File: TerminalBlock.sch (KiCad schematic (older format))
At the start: 2 parts, among them P4 12 Pin Terminal Block, P5 3 Pin TB

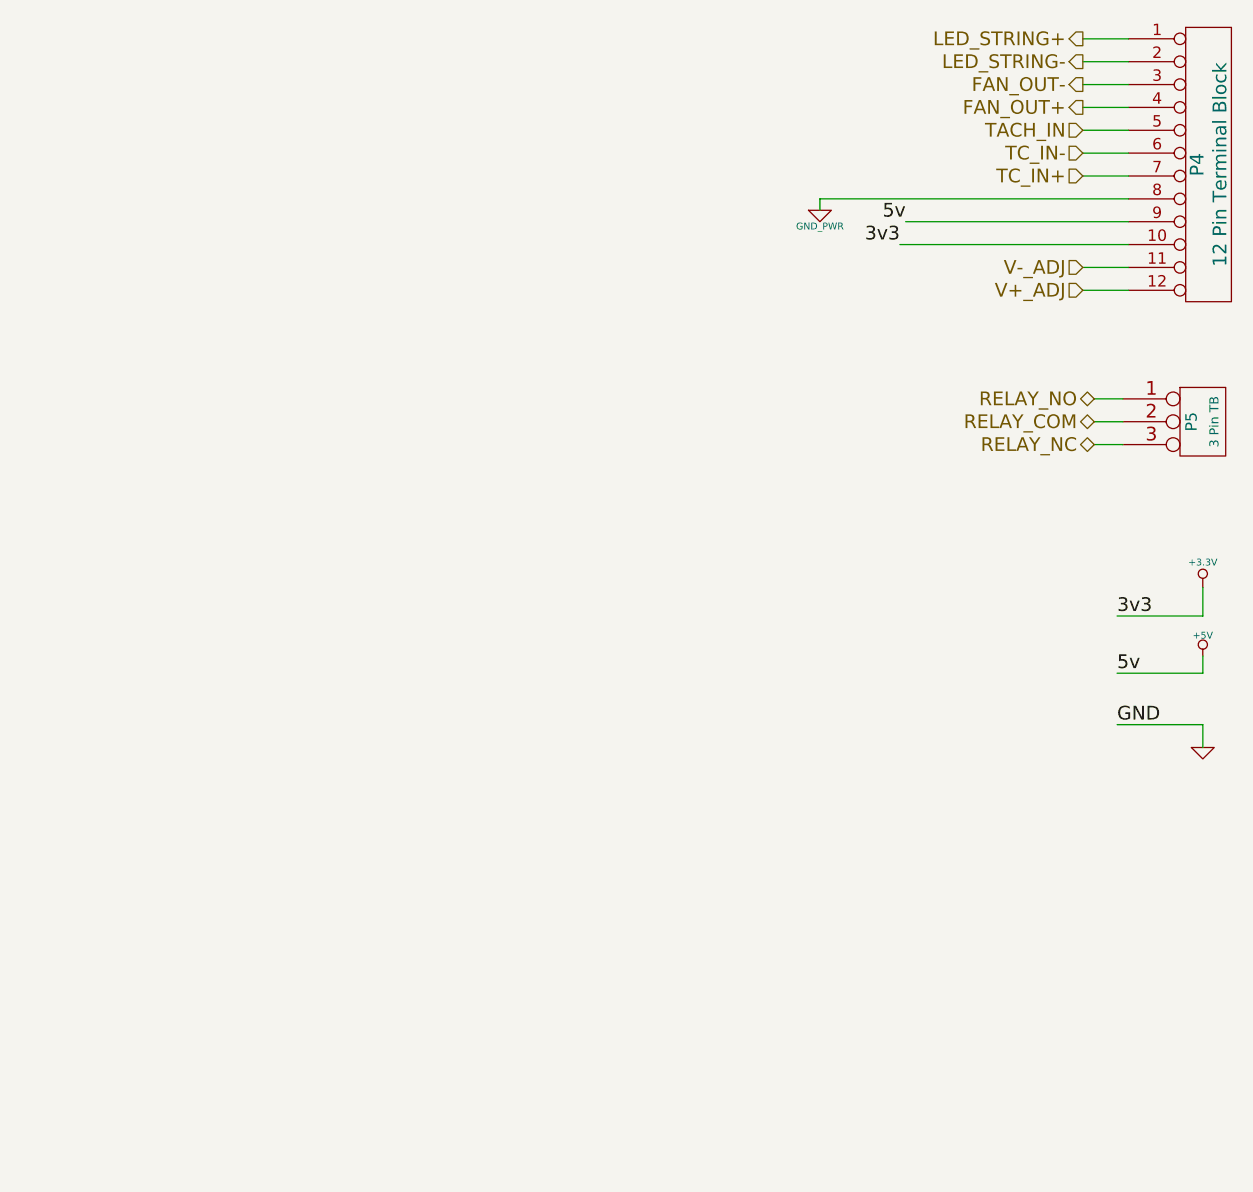
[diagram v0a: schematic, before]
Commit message: Layout Work Session 6
Pulled from CE
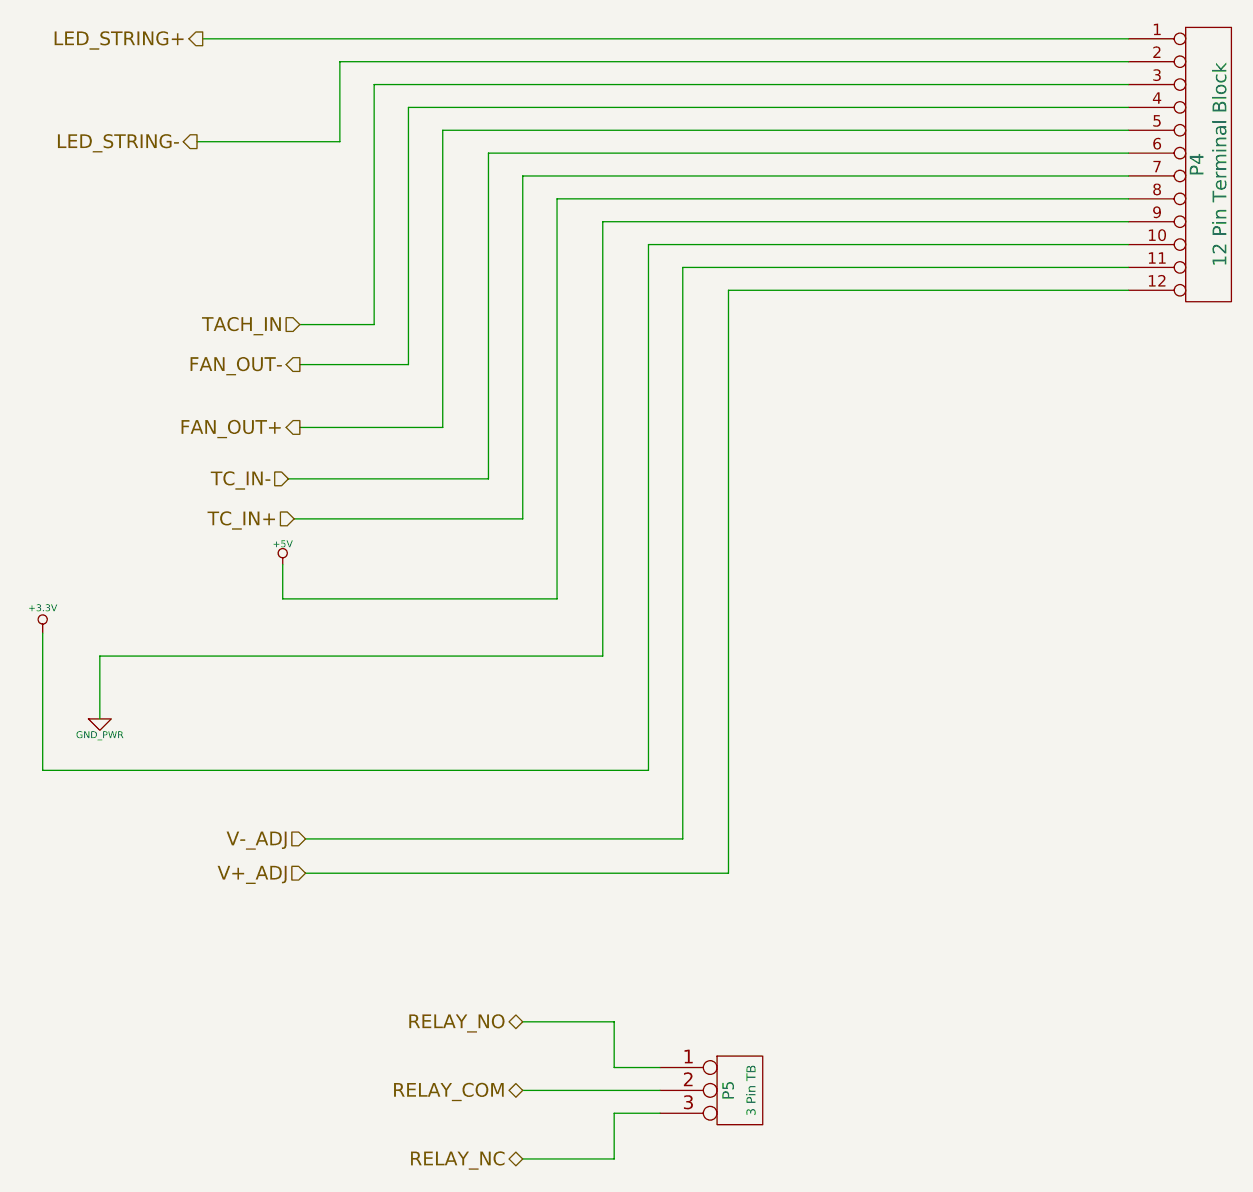
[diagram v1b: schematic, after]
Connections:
- net +5V: now also P4.8 (P8); no longer P4.9 (P9)
- net FAN_OUT+: now also P4.5 (P5); no longer P4.4 (P4)
- net FAN_OUT-: now also P4.4 (P4); no longer P4.3 (P3)
- net GND_PWR: now also P4.9 (P9); no longer P4.8 (P8)
- net TACH_IN: now also P4.3 (P3); no longer P4.5 (P5)
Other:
- moved on the sheet: P5
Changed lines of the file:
@@
-EESchema Schematic File Version 2
+EESchema Schematic File Version 2  date 11/10/2013 9:27:17 PM
 LIBS:power
 LIBS:device
@@
 LIBS:valves
 LIBS:BenchBuddy
-LIBS:arduino_shieldsNCL
 LIBS:BenchBuddy-cache
-EELAYER 24 0
+EELAYER 27 0
 EELAYER END
 $Descr A4 11693 8268
@@
 Sheet 7 9
 Title ""
-Date "2 nov 2013"
+Date "11 nov 2013"
 Rev ""
 Comp ""
@@
 Comment4 ""
 $EndDescr
-Text HLabel 5300 2000 0    60   Input ~ 0
+Text HLabel 1900 4550 0    60   Input ~ 0
 V+_ADJ
-Text HLabel 5300 1900 0    60   Input ~ 0
+Text HLabel 1900 4400 0    60   Input ~ 0
 V-_ADJ
-Text HLabel 5300 1200 0    60   Output ~ 0
+Text HLabel 1875 2600 0    60   Output ~ 0
 FAN_OUT+
-Text HLabel 5300 1100 0    60   Output ~ 0
+Text HLabel 1875 2325 0    60   Output ~ 0
 FAN_OUT-
-Text HLabel 5300 1300 0    60   Input ~ 0
+Text HLabel 1875 2150 0    60   Input ~ 0
 TACH_IN
-Text HLabel 5300 900  0    60   Output ~ 0
+Text HLabel 1450 900  0    60   Output ~ 0
 LED_STRING+
-Text HLabel 5300 1000 0    60   Output ~ 0
+Text HLabel 1425 1350 0    60   Output ~ 0
 LED_STRING-
-Text HLabel 5300 1500 0    60   Input ~ 0
+Text HLabel 1850 3000 0    60   Input ~ 0
 TC_IN+
-Text HLabel 5300 1400 0    60   Input ~ 0
+Text HLabel 1825 2825 0    60   Input ~ 0
 TC_IN-
-Text HLabel 5350 2575 0    60   BiDi ~ 0
+Text HLabel 2850 5500 0    60   BiDi ~ 0
 RELAY_COM
-Text HLabel 5350 2475 0    60   BiDi ~ 0
+Text HLabel 2850 5200 0    60   BiDi ~ 0
 RELAY_NO
-Text HLabel 5350 2675 0    60   BiDi ~ 0
+Text HLabel 2850 5800 0    60   BiDi ~ 0
 RELAY_NC
 $Comp
-L +3.3V #PWR038
+L +3.3V #PWR44
 U 1 1 523FFDA7
-P 5825 3300
-F 0 "#PWR038" H 5825 3260 30  0001 C CNN
-F 1 "+3.3V" H 5825 3410 30  0000 C CNN
-F 2 "~" H 5825 3300 60  0000 C CNN
-F 3 "~" H 5825 3300 60  0000 C CNN
-	1    5825 3300
-	1    0    0    -1
-$EndComp
-$Comp
-L +5V #PWR039
+P 750 3500
+F 0 "#PWR44" H 750 3460 30  0001 C CNN
+F 1 "+3.3V" H 750 3610 30  0000 C CNN
+F 2 "~" H 750 3500 60  0000 C CNN
+F 3 "~" H 750 3500 60  0000 C CNN
+	1    750  3500
+	1    0    0    -1
+$EndComp
+$Comp
+L +5V #PWR45
 U 1 1 523FFDB6
-P 5825 3600
-F 0 "#PWR039" H 5825 3690 20  0001 C CNN
-F 1 "+5V" H 5825 3690 30  0000 C CNN
-F 2 "~" H 5825 3600 60  0000 C CNN
-F 3 "~" H 5825 3600 60  0000 C CNN
-	1    5825 3600
+P 1800 3200
+F 0 "#PWR45" H 1800 3290 20  0001 C CNN
+F 1 "+5V" H 1800 3290 30  0000 C CNN
+F 2 "~" H 1800 3200 60  0000 C CNN
+F 3 "~" H 1800 3200 60  0000 C CNN
+	1    1800 3200
 	1    0    0    -1
 $EndComp
@@
 	1    0    0    -1
 $EndComp
+Wire Wire Line
+	1425 1350 2050 1350
+Wire Wire Line
+	2050 1350 2050 1000
+Wire Wire Line
+	2050 1000 5500 1000
+Wire Wire Line
+	2200 1100 5500 1100
+Wire Wire Line
+	2200 1100 2200 2150
+Wire Wire Line
+	2350 1200 2350 2325
+Wire Wire Line
+	2350 1200 5500 1200
+Wire Wire Line
+	5500 1300 2500 1300
+Wire Wire Line
+	2500 1300 2500 2600
+Wire Wire Line
+	2700 2825 2700 1400
+Wire Wire Line
+	2700 1400 5500 1400
+Wire Wire Line
+	1800 3350 3000 3350
+Wire Wire Line
+	1000 3600 3200 3600
+Wire Wire Line
+	750  4100 3400 4100
+Wire Wire Line
+	2850 1500 2850 3000
+Wire Wire Line
+	2850 1500 5500 1500
+Wire Wire Line
+	5500 1600 3000 1600
+Wire Wire Line
+	3000 1600 3000 3350
+Wire Wire Line
+	3200 3600 3200 1700
+Wire Wire Line
+	3200 1700 5500 1700
+Wire Wire Line
+	5500 1800 3400 1800
+Wire Wire Line
+	3400 1800 3400 4100
+Wire Wire Line
+	1900 4400 3550 4400
+Wire Wire Line
+	3550 4400 3550 1900
+Wire Wire Line
+	3550 1900 5500 1900
+Wire Wire Line
+	5500 2000 3750 2000
+Wire Wire Line
+	3750 2000 3750 4550
+Wire Wire Line
+	3750 4550 1900 4550
 $Comp
 L CONN_3 P5
 U 1 1 5258AA07
-P 5825 2575
-F 0 "P5" V 5775 2575 50  0000 C CNN
-F 1 "3 Pin TB" V 5875 2575 40  0000 C CNN
-F 2 "" H 5825 2575 60  0000 C CNN
-F 3 "" H 5825 2575 60  0000 C CNN
-F 4 "Phoenix" H 5825 2575 60  0001 C CNN "MFG Name"
-F 5 "1935174" H 5825 2575 60  0001 C CNN "MFG Part Number"
-	1    5825 2575
-	1    0    0    -1
-$EndComp
-Wire Wire Line
-	5475 2575 5350 2575
-$Comp
-L GND #PWR040
-U 1 1 523FFDC5
-P 5825 4000
-F 0 "#PWR040" H 5825 4000 30  0001 C CNN
-F 1 "GND" H 5825 3930 30  0001 C CNN
-F 2 "~" H 5825 4000 60  0000 C CNN
-F 3 "~" H 5825 4000 60  0000 C CNN
-	1    5825 4000
-	1    0    0    -1
-$EndComp
-Wire Wire Line
-	5350 2475 5475 2475
-Wire Wire Line
-	5350 2675 5475 2675
-Wire Wire Line
-	5825 3300 5825 3425
-Wire Wire Line
-	5825 3425 5450 3425
-Text Label 5450 3425 0    60   ~ 0
-3v3
-Wire Wire Line
-	5825 3600 5825 3675
-Wire Wire Line
-	5825 3675 5450 3675
-Wire Wire Line
-	5825 4000 5825 3900
-Wire Wire Line
-	5825 3900 5450 3900
-Text Label 5450 3675 0    60   ~ 0
-5v
-Text Label 5450 3900 0    60   ~ 0
-GND
-Wire Wire Line
-	5300 2000 5500 2000
-Wire Wire Line
-	5500 1900 5300 1900
-Wire Wire Line
-	4500 1800 5500 1800
-Wire Wire Line
-	4525 1700 5500 1700
-Wire Wire Line
-	4150 1600 5500 1600
-Wire Wire Line
-	5500 1300 5300 1300
-Wire Wire Line
-	5500 900  5300 900
-Wire Wire Line
-	5300 1000 5500 1000
-Wire Wire Line
-	5500 1200 5300 1200
-Wire Wire Line
-	5500 1100 5300 1100
-Wire Wire Line
-	5500 1400 5300 1400
-Wire Wire Line
-	5500 1500 5300 1500
-Text Label 4500 1800 2    60   ~ 0
-3v3
-Text Label 4525 1700 2    60   ~ 0
-5v
-$Comp
-L GND_PWR #PWR041
-U 1 1 5314831E
-P 4150 1650
-F 0 "#PWR041" H 4150 1650 30  0001 C CNN
-F 1 "GND_PWR" H 4150 1580 30  0000 C CNN
-F 2 "" H 4150 1650 60  0000 C CNN
-F 3 "" H 4150 1650 60  0000 C CNN
-	1    4150 1650
-	1    0    0    -1
-$EndComp
-Wire Wire Line
-	4150 1650 4150 1600
+P 3800 5500
+F 0 "P5" V 3750 5500 50  0000 C CNN
+F 1 "3 Pin TB" V 3850 5500 40  0000 C CNN
+F 2 "" H 3800 5500 60  0000 C CNN
+F 3 "" H 3800 5500 60  0000 C CNN
+F 4 "Phoenix" H 3800 5500 60  0001 C CNN "MFG Name"
+F 5 "1935174" H 3800 5500 60  0001 C CNN "MFG Part Number"
+	1    3800 5500
+	1    0    0    -1
+$EndComp
+Wire Wire Line
+	3450 5500 2850 5500
+Wire Wire Line
+	2850 5200 3250 5200
+Wire Wire Line
+	3250 5200 3250 5400
+Wire Wire Line
+	3250 5400 3450 5400
+Wire Wire Line
+	3450 5600 3250 5600
+Wire Wire Line
+	3250 5600 3250 5800
+Wire Wire Line
+	3250 5800 2850 5800
+Wire Wire Line
+	750  4100 750  3500
+Wire Wire Line
+	2850 3000 1850 3000
+Wire Wire Line
+	2350 2325 1875 2325
+Wire Wire Line
+	2500 2600 1875 2600
+Wire Wire Line
+	2200 2150 1875 2150
+Wire Wire Line
+	1825 2825 2700 2825
+Wire Wire Line
+	1450 900  5500 900
+$Comp
+L GND_PWR #PWR46
+U 1 1 527EF77D
+P 1000 3875
+F 0 "#PWR46" H 1000 3875 30  0001 C CNN
+F 1 "GND_PWR" H 1000 3805 30  0000 C CNN
+F 2 "~" H 1000 3875 60  0000 C CNN
+F 3 "~" H 1000 3875 60  0000 C CNN
+	1    1000 3875
+	1    0    0    -1
+$EndComp
+Wire Wire Line
+	1000 3600 1000 3875
+Wire Wire Line
+	1800 3200 1800 3350
 $EndSCHEMATC
